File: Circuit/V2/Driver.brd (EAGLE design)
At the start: 58.8 x 53.6 mm, 36 parts

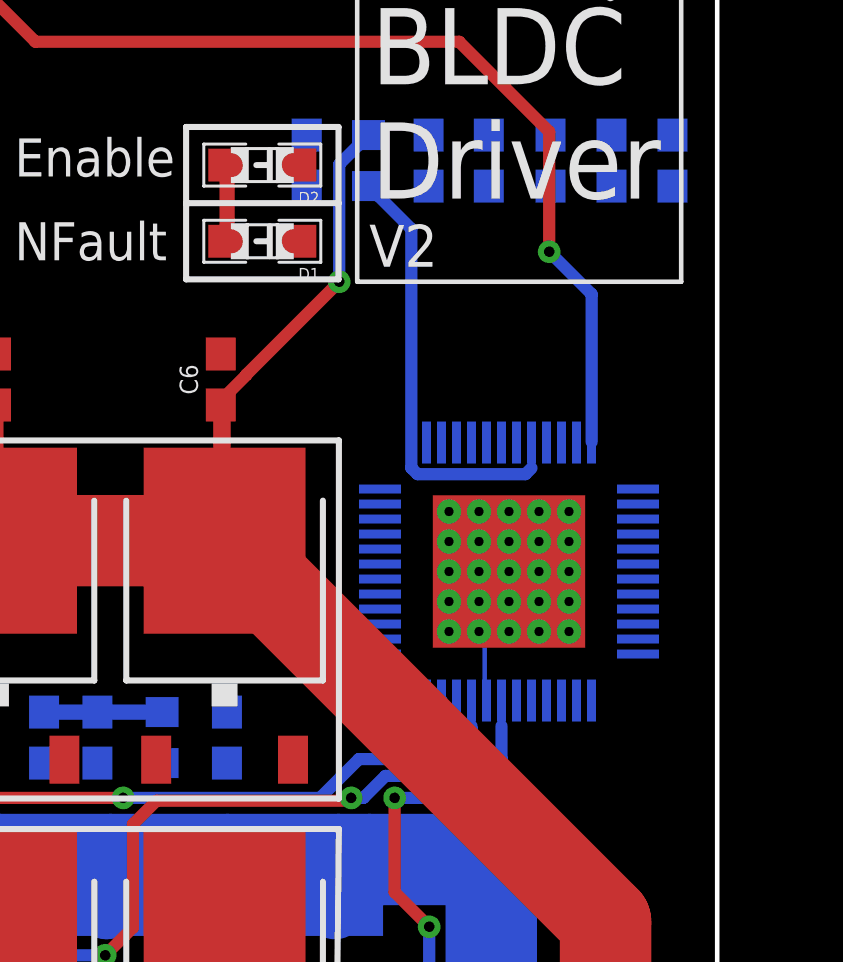
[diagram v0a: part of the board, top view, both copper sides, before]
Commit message: Fix some routering bug
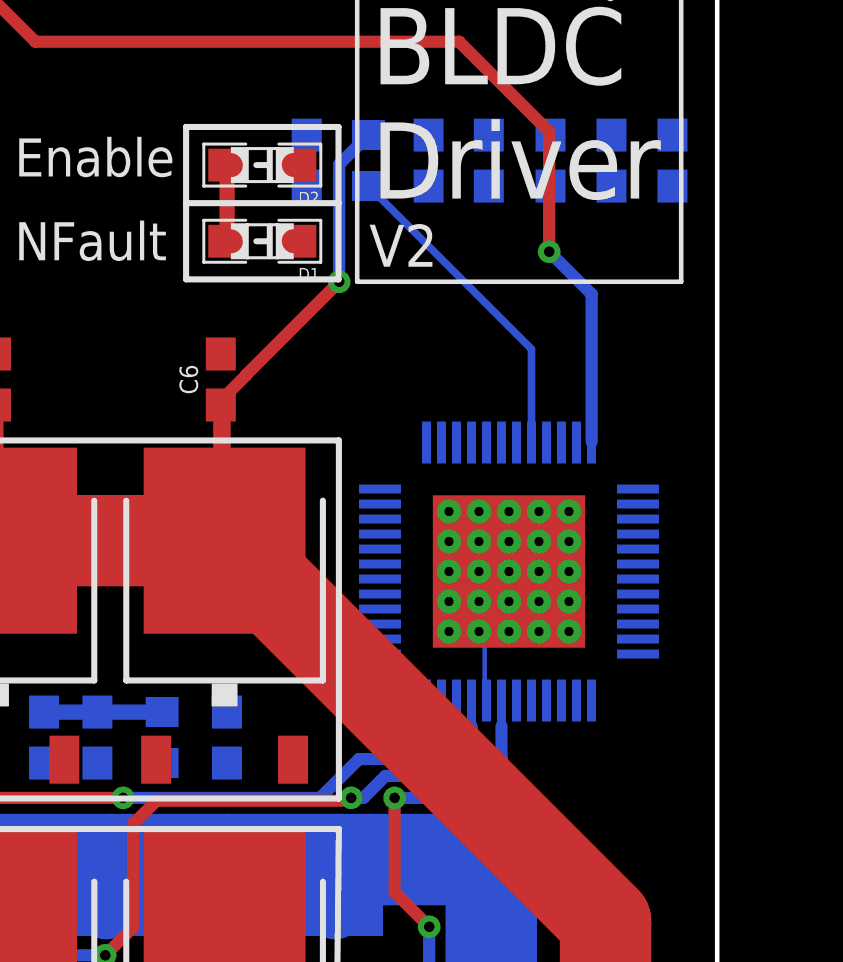
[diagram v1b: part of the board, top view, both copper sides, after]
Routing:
- net VDRAIN: track 14.2 -> 10.8 mm
- net SN2: track 22.0 -> 22.9 mm
- net SN3: track 19.9 -> 20.8 mm
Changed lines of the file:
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@@
 <drawing>
 <settings>
-<setting alwaysvectorfont="yes"/>
+<setting alwaysvectorfont="no"/>
 <setting verticaltext="up"/>
 </settings>
@@
 <wire x1="53.66" y1="23.84" x2="54.66" y2="23.84" width="0.1524" layer="1"/>
 <wire x1="56.077" y1="37.688" x2="58.109" y2="39.388" width="0" layer="19" extent="16-16"/>
-<wire x1="49.981" y1="39.388" x2="56.077" y2="37.688" width="0" layer="19" extent="16-16"/>
+<wire x1="56.077" y1="37.688" x2="49.981" y2="39.388" width="0" layer="19" extent="16-16"/>
 <wire x1="43.262" y1="38.389" x2="49.981" y2="39.388" width="0" layer="19" extent="1-16"/>
 <wire x1="43.053" y1="32.092" x2="43.262" y2="35.849" width="0" layer="19" extent="1-1"/>
@@
 <wire x1="48.84775625" y1="17.2946" x2="51.0946" y2="17.2946" width="0.4064" layer="16"/>
 <wire x1="51.0946" y1="17.2946" x2="52.41" y2="18.61" width="0.4064" layer="16"/>
-<wire x1="52.41" y1="19.68710625" x2="52.41" y2="20.54" width="0" layer="19" extent="16-16"/>
+<wire x1="52.41" y1="19.68710625" x2="52.41" y2="20.54" width="0.3" layer="16"/>
+<wire x1="52.41" y1="20.54" x2="48.36" y2="22.59" width="0" layer="19" extent="16-16"/>
+<wire x1="47.5" y1="4.5" x2="46.5" y2="4.5" width="0" layer="19" extent="1-1"/>
+<wire x1="46.5" y1="3.5" x2="46.5" y2="4.5" width="0" layer="19" extent="1-1"/>
+<wire x1="47.5" y1="3.5" x2="47.5" y2="4.5" width="0" layer="19" extent="1-1"/>
+<wire x1="45.5" y1="4.5" x2="46.5" y2="4.5" width="0" layer="19" extent="1-1"/>
+<wire x1="45.5" y1="3.5" x2="46.5" y2="3.5" width="0" layer="19" extent="1-1"/>
+<wire x1="46.5" y1="2.5" x2="46.5" y2="3.5" width="0" layer="19" extent="1-1"/>
+<wire x1="47.5" y1="2.5" x2="47.5" y2="3.5" width="0" layer="19" extent="1-1"/>
+<wire x1="45.5" y1="2.5" x2="45.5" y2="3.5" width="0" layer="19" extent="1-1"/>
+<wire x1="45.46" y1="5.868" x2="45.5" y2="4.5" width="0" layer="19" extent="1-1"/>
+<wire x1="46.863" y1="7.995" x2="45.46" y2="5.868" width="0" layer="19" extent="1-16"/>
 <wire x1="43.18" y1="9.945" x2="46.863" y2="7.995" width="0" layer="19" extent="16-16"/>
-<wire x1="48.36" y1="22.59" x2="52.41" y2="20.54" width="0" layer="19" extent="16-16"/>
 </signal>
 <signal name="SH_C">
@@
 <wire x1="47.81000625" y1="17.2946" x2="47.4" y2="17.2946" width="0.4064" layer="16"/>
 <wire x1="48.54380625" y1="18.0284" x2="47.81000625" y2="17.2946" width="0.4064" layer="16"/>
-<wire x1="51.41" y1="19.61" x2="49.8284" y2="18.0284" width="0.4064" layer="16"/>
+<wire x1="49.8284" y1="18.0284" x2="51.41" y2="19.61" width="0.4064" layer="16"/>
 <wire x1="49.8284" y1="18.0284" x2="48.54380625" y2="18.0284" width="0.4064" layer="16"/>
 <wire x1="47.4" y1="17.2946" x2="47.3054" y2="17.2" width="0.4064" layer="1"/>
 <wire x1="47.3054" y1="17.2" x2="40.90910625" y2="17.2" width="0.4064" layer="1"/>
-<wire x1="51.41" y1="19.68710625" x2="51.41" y2="20.54" width="0" layer="19" extent="16-16"/>
+<wire x1="51.41" y1="19.61" x2="51.41" y2="20.54" width="0.3" layer="16"/>
+<wire x1="51.41" y1="20.54" x2="48.36" y2="25.09" width="0" layer="19" extent="16-16"/>
 <wire x1="39.243" y1="7.995" x2="39.2" y2="12.0484" width="0" layer="19" extent="16-16"/>
-<wire x1="48.36" y1="25.09" x2="51.41" y2="20.54" width="0" layer="19" extent="16-16"/>
+<wire x1="37.84" y1="5.868" x2="39.243" y2="7.995" width="0" layer="19" extent="1-16"/>
+<wire x1="38" y1="4.5" x2="37.84" y2="5.868" width="0" layer="19" extent="1-1"/>
+<wire x1="39" y1="4.5" x2="38" y2="4.5" width="0" layer="19" extent="1-1"/>
+<wire x1="40" y1="4.5" x2="39" y2="4.5" width="0" layer="19" extent="1-1"/>
+<wire x1="39" y1="3.5" x2="39" y2="4.5" width="0" layer="19" extent="1-1"/>
+<wire x1="40" y1="3.5" x2="40" y2="4.5" width="0" layer="19" extent="1-1"/>
+<wire x1="38" y1="3.5" x2="38" y2="4.5" width="0" layer="19" extent="1-1"/>
+<wire x1="39" y1="2.5" x2="39" y2="3.5" width="0" layer="19" extent="1-1"/>
+<wire x1="40" y1="2.5" x2="40" y2="3.5" width="0" layer="19" extent="1-1"/>
+<wire x1="38" y1="2.5" x2="38" y2="3.5" width="0" layer="19" extent="1-1"/>
 </signal>
 <signal name="GL_B">
@@
 <contactref element="U$3" pad="44"/>
 <contactref element="R4" pad="1"/>
-<wire x1="49.4044" y1="28.29270625" x2="49.61270625" y2="28.0844" width="0.4064" layer="16"/>
-<wire x1="53.20729375" y1="28.0844" x2="53.41" y2="28.28710625" width="0.4064" layer="16"/>
-<wire x1="49.61270625" y1="28.0844" x2="53.20729375" y2="28.0844" width="0.4064" layer="16"/>
-<wire x1="47.977" y1="37.688" x2="49.4044" y2="36.2606" width="0.4064" layer="16"/>
-<wire x1="49.4044" y1="36.2606" x2="49.4044" y2="28.29270625" width="0.4064" layer="16"/>
-<wire x1="53.41" y1="28.28710625" x2="53.41" y2="29.14" width="0" layer="19" extent="16-16"/>
+<wire x1="47.977" y1="37.688" x2="53.41" y2="32.255" width="0.254" layer="16"/>
+<wire x1="53.41" y1="32.255" x2="53.41" y2="29.14" width="0.254" layer="16"/>
 </signal>
 <signal name="DVDD">
@@
 <wire x1="32.5044" y1="16.41529375" x2="33.38370625" y2="17.2946" width="0.4064" layer="1"/>
 <wire x1="33.38370625" y1="17.2946" x2="39.8" y2="17.2946" width="0.4064" layer="1"/>
-<wire x1="50.41" y1="20.54" x2="50.4" y2="20.53" width="0.4064" layer="16"/>
-<wire x1="50.4" y1="20.53" x2="50.4" y2="19.4" width="0.4064" layer="16"/>
+<wire x1="50.41" y1="20.54" x2="50.4" y2="20.53" width="0.3" layer="16"/>
+<wire x1="50.4" y1="20.53" x2="50.4" y2="19.4" width="0.3" layer="16"/>
 <wire x1="50.4" y1="19.4" x2="49.5872" y2="18.5872" width="0.4064" layer="16"/>
 <wire x1="49.5872" y1="18.5872" x2="47.65485" y2="18.5872" width="0.4064" layer="16"/>
@@
 <wire x1="50.41" y1="20.54" x2="48.36" y2="26.59" width="0" layer="19" extent="16-16"/>
 <wire x1="31.623" y1="7.995" x2="31.6" y2="12" width="0" layer="19" extent="16-16"/>
+<wire x1="31.5" y1="4.5" x2="30.5" y2="4.5" width="0" layer="19" extent="1-1"/>
+<wire x1="32.5" y1="4.5" x2="31.5" y2="4.5" width="0" layer="19" extent="1-1"/>
+<wire x1="30.5" y1="3.5" x2="30.5" y2="4.5" width="0" layer="19" extent="1-1"/>
+<wire x1="31.5" y1="3.5" x2="31.5" y2="4.5" width="0" layer="19" extent="1-1"/>
+<wire x1="32.5" y1="3.5" x2="32.5" y2="4.5" width="0" layer="19" extent="1-1"/>
+<wire x1="30.5" y1="2.5" x2="30.5" y2="3.5" width="0" layer="19" extent="1-1"/>
+<wire x1="31.5" y1="2.5" x2="31.5" y2="3.5" width="0" layer="19" extent="1-1"/>
+<wire x1="32.5" y1="2.5" x2="32.5" y2="3.5" width="0" layer="19" extent="1-1"/>
 </signal>
 <signal name="PWRGD">
